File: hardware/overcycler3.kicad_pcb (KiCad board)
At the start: 2 copper layers, 200.7 x 99.1 mm, 308 parts, among them IC1 LM13700, IC2 LM13700, IC3 LM13700, J1 USB_B, J2 AudioJack3_Switch, J3 DIN-5_180degree, J4 AudioJack3_Switch, J5 AudioJack3_Switch, P1 FT232, P2 PANEL, Q1 2SC945, SW1 RESET, SW2 POWER, U1 XT26G02ELGIGA, U10 MCP4922-ESL, U11 SSI2144, U12 MCP4922-ESL, U13 SSI2144, U14 MCP4922-ESL, U15 SSI2144, U16 MCP4922-ESL, U17 SSI2144, U18 MCP4922-ESL, U19 SSI2144, U2 TL074, U20 AD5328B, U3 LPC1778FBD144, U4 TLV2556, U5 74HC138, U6 TL074, U7 AD5328B, U8 MCP4922-ESL, U9 SSI2144, Y1 12MHz

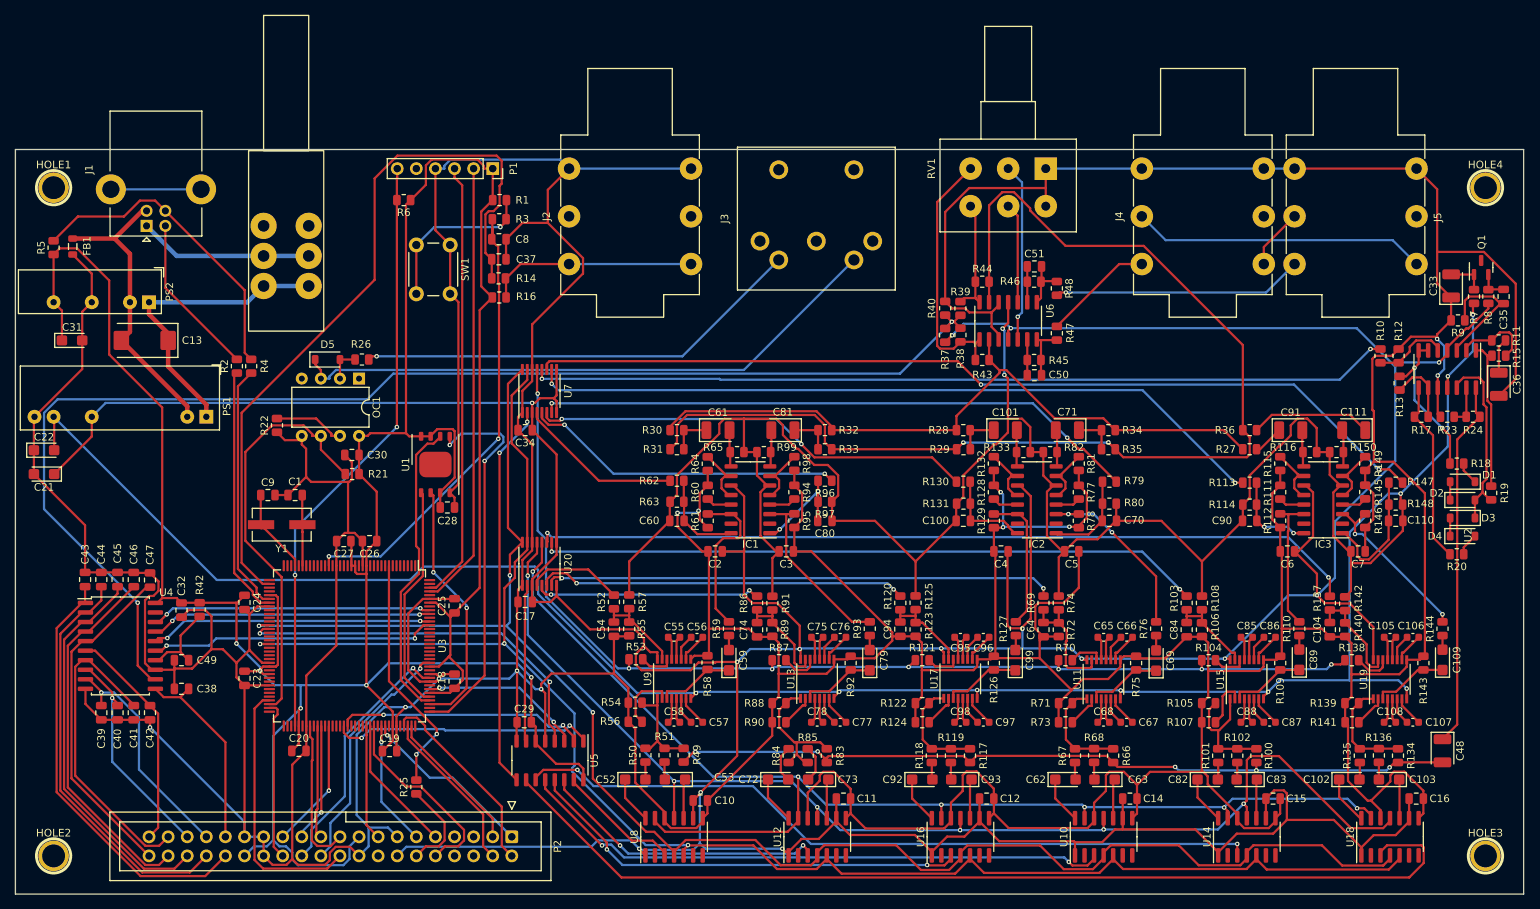
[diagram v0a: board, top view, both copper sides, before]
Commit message: hardware: chnaged some capacitor values and footprints
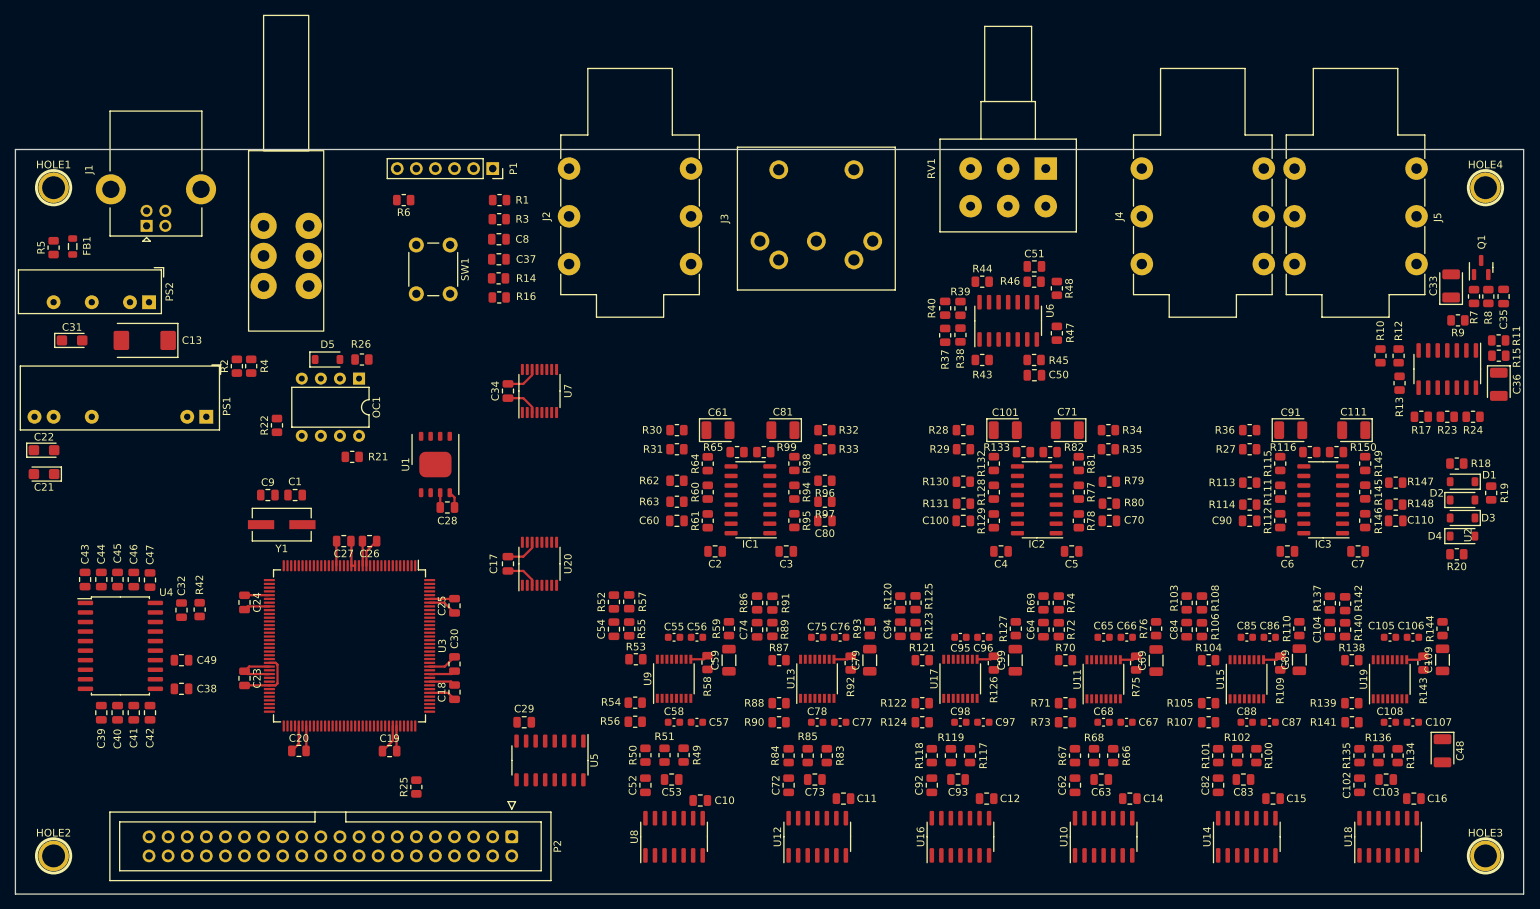
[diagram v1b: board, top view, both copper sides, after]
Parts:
- C102, C103, C52, C53, C62, C63, C72, C73, C82, C83, C92, C93: footprint Capacitor_Tantalum_SMD:CP_EIA-3216-18_Kemet-A -> Capacitor_SMD:C_0805_2012Metric
- C109, C59, C69, C79, C89, C99: value 33u -> 47u; footprint Capacitor_Tantalum_SMD:CP_EIA-3216-18_Kemet-A -> Capacitor_SMD:C_1206_3216Metric
- moved C30 31.0 mm to (78.7, 106.5), turned to -90 degrees
- moved C34 5.69 mm to (85.9, 70.2), turned to 90 degrees
- moved C17 5.57 mm to (85.9, 93.2), turned to 90 degrees
- moved R21 2.29 mm to (65.1, 79.0)
- moved C72 1.59 mm to (123.2, 122.7), turned to 90 degrees
- moved C82 1.59 mm to (180.3, 122.7), turned to 90 degrees
- moved C102 1.55 mm to (199.1, 122.7), turned to 90 degrees
- moved C52 1.55 mm to (104.1, 122.7), turned to 90 degrees
- moved C92 1.48 mm to (142.2, 122.7), turned to 90 degrees
- moved C62 1.48 mm to (161.3, 122.7), turned to 90 degrees
- moved C18 1.46 mm to (78.7, 110.3)
- moved C53 0.45 mm to (107.6, 121.9)
- moved C63 0.45 mm to (164.8, 121.9)
- moved C83 0.45 mm to (183.7, 121.9)
- moved C93 0.45 mm to (145.7, 121.9)
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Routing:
- net GND: track 1285.8 -> 60.6 mm, vias 12 -> 0
- net +5V: track 655.5 -> 8.94 mm, vias 14 -> 0
- net -5V: track 539.0 -> 0.00 mm, vias 11 -> 0
- net +3.3V: track 419.4 -> 38.9 mm, vias 5 -> 0
- net SPI_SCK: track 221.2 -> 0.00 mm, vias 3 -> 0
- net SPI_MOSI: track 219.6 -> 0.00 mm, vias 3 -> 0
- net /ADC_MIX: track 172.9 -> 0.00 mm, vias 2 -> 0
- net DAC_MIXA: track 164.1 -> 0.00 mm, vias 6 -> 0
- net DAC_MIXB: track 161.9 -> 0.00 mm, vias 6 -> 0
- net Net-(U6D--): track 155.8 -> 0.00 mm, vias 2 -> 0
- net DAC_RES: track 147.8 -> 0.00 mm, vias 7 -> 0
- net /SPI_CS5: track 134.6 -> 0.00 mm
- net /DAC_VCA5: track 121.5 -> 0.00 mm, vias 2 -> 0
- net /DAC_MIXN: track 114.5 -> 0.00 mm, vias 2 -> 0
- net /DAC_FC5: track 110.2 -> 0.00 mm, vias 2 -> 0
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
